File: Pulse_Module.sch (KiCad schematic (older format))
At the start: 6 parts, among them CON3 BARREL_JACK, U3 AP1117

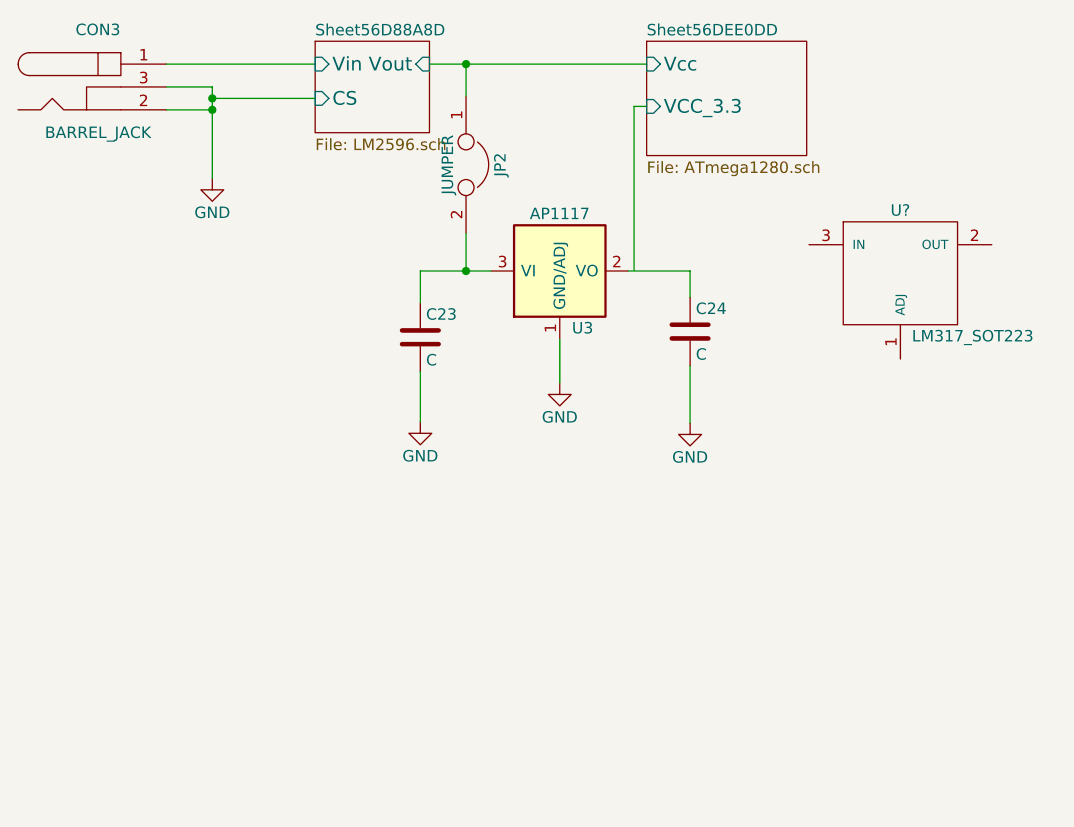
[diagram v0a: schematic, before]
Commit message: Изменения футпринтов
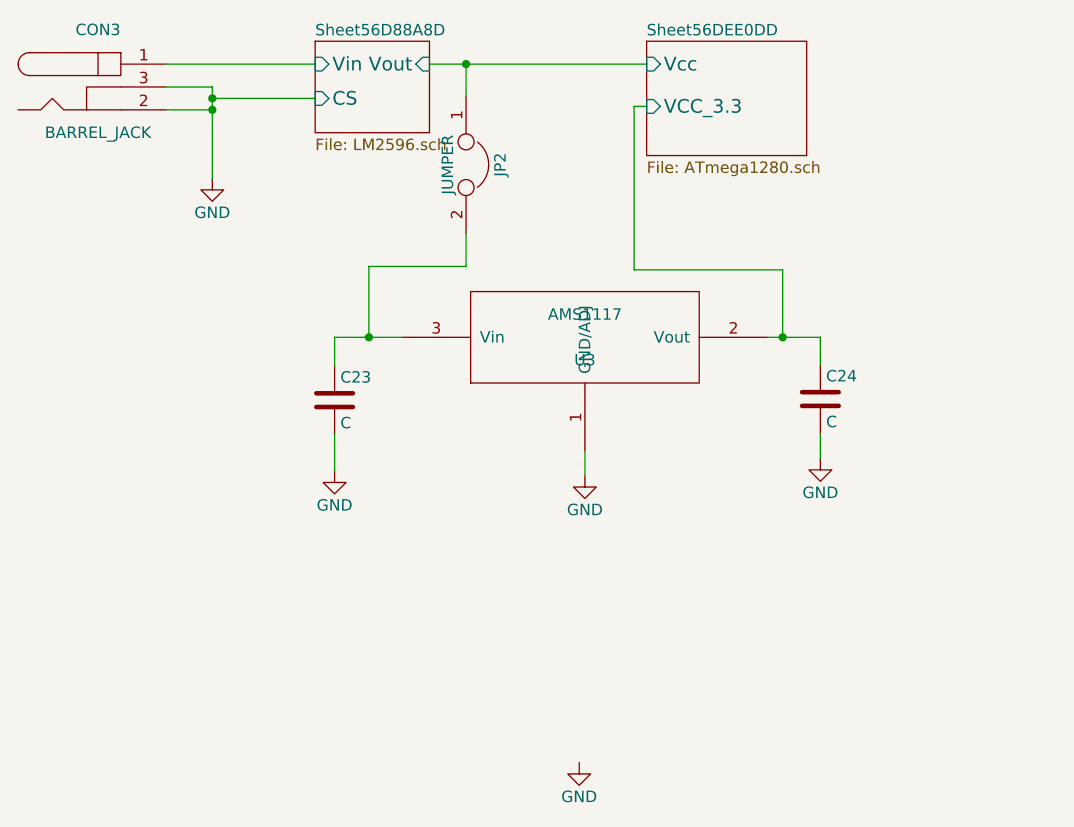
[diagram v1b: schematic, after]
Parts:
- removed U3: AP1117, TO_SOT_Packages_SMD:TO-252-2Lead, symbol AP1117
- removed U?: LM317_SOT223, symbol LM317_SOT223
- added U3: AMS1117, TO_SOT_Packages_SMD:TO-252-2Lead, symbol AMS1117
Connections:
- wire segments 17 -> 21
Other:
- moved on the sheet: C23, C24
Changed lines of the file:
@@
 LIBS:contrib
 LIBS:valves
+LIBS:AMS1117
 LIBS:Pulse_Module-cache
 EELAYER 25 0
@@
 $EndComp
 $Comp
-L AP1117 U3
-U 1 1 57F2F385
-P 4070 4655
-F 0 "U3" H 4170 4405 50  0000 C CNN
-F 1 "AP1117" H 4070 4905 50  0000 C CNN
-F 2 "TO_SOT_Packages_SMD:TO-252-2Lead" H 4070 4655 50  0001 C CNN
-F 3 "" H 4070 4655 50  0000 C CNN
-	1    4070 4655
-	1    0    0    -1
-$EndComp
-$Comp
-L C C23
-U 1 1 57F2F689
-P 3460 4945
-F 0 "C23" H 3485 5045 50  0000 L CNN
-F 1 "C" H 3485 4845 50  0000 L CNN
-F 2 "Capacitors_SMD:C_0805" H 3498 4795 50  0001 C CNN
-F 3 "" H 3460 4945 50  0000 C CNN
-	1    3460 4945
-	1    0    0    -1
-$EndComp
-$Comp
 L C C24
 U 1 1 57F2F6D4
-P 4640 4920
-F 0 "C24" H 4665 5020 50  0000 L CNN
-F 1 "C" H 4665 4820 50  0000 L CNN
-F 2 "Capacitors_SMD:C_0805" H 4678 4770 50  0001 C CNN
-F 3 "" H 4640 4920 50  0000 C CNN
-	1    4640 4920
+P 5210 5215
+F 0 "C24" H 5235 5315 50  0000 L CNN
+F 1 "C" H 5235 5115 50  0000 L CNN
+F 2 "Capacitors_SMD:C_0805" H 5248 5065 50  0001 C CNN
+F 3 "" H 5210 5215 50  0000 C CNN
+	1    5210 5215
 	1    0    0    -1
 $EndComp
@@
 L GND #PWR02
 U 1 1 57F2F7B1
-P 3460 5315
-F 0 "#PWR02" H 3460 5065 50  0001 C CNN
-F 1 "GND" H 3460 5165 50  0000 C CNN
-F 2 "" H 3460 5315 50  0000 C CNN
-F 3 "" H 3460 5315 50  0000 C CNN
-	1    3460 5315
+P 4180 5550
+F 0 "#PWR02" H 4180 5300 50  0001 C CNN
+F 1 "GND" H 4180 5400 50  0000 C CNN
+F 2 "" H 4180 5550 50  0000 C CNN
+F 3 "" H 4180 5550 50  0000 C CNN
+	1    4180 5550
 	1    0    0    -1
 $EndComp
@@
 L GND #PWR03
 U 1 1 57F2F900
-P 4640 5320
-F 0 "#PWR03" H 4640 5070 50  0001 C CNN
-F 1 "GND" H 4640 5170 50  0000 C CNN
-F 2 "" H 4640 5320 50  0000 C CNN
-F 3 "" H 4640 5320 50  0000 C CNN
-	1    4640 5320
+P 5210 5475
+F 0 "#PWR03" H 5210 5225 50  0001 C CNN
+F 1 "GND" H 5210 5325 50  0000 C CNN
+F 2 "" H 5210 5475 50  0000 C CNN
+F 3 "" H 5210 5475 50  0000 C CNN
+	1    5210 5475
 	1    0    0    -1
 $EndComp
@@
 L GND #PWR04
 U 1 1 57F30351
-P 4070 5145
-F 0 "#PWR04" H 4070 4895 50  0001 C CNN
-F 1 "GND" H 4070 4995 50  0000 C CNN
-F 2 "" H 4070 5145 50  0000 C CNN
-F 3 "" H 4070 5145 50  0000 C CNN
-	1    4070 5145
+P 4155 6805
+F 0 "#PWR04" H 4155 6555 50  0001 C CNN
+F 1 "GND" H 4155 6655 50  0000 C CNN
+F 2 "" H 4155 6805 50  0000 C CNN
+F 3 "" H 4155 6805 50  0000 C CNN
+	1    4155 6805
 	1    0    0    -1
 $EndComp
@@
 Wire Wire Line
 	3500 3750 4450 3750
-Wire Wire Line
-	4640 5070 4640 5320
-Wire Wire Line
-	3460 5095 3460 5315
-Connection ~ 3660 4655
 Connection ~ 3660 3750
 Wire Wire Line
-	4070 4955 4070 5145
-Wire Wire Line
-	4370 4655 4640 4655
-Wire Wire Line
-	4640 4655 4640 4770
-Wire Wire Line
-	4395 4650 4395 3935
-Wire Wire Line
 	3660 3750 3660 3890
-Wire Wire Line
-	3460 4655 3460 4795
 $Sheet
 S 4450 3650 700  500
@@
 Wire Wire Line
 	4395 3935 4450 3935
-Wire Wire Line
-	3460 4655 3770 4655
-Wire Wire Line
-	3660 4490 3660 4655
 $Comp
-L LM317_SOT223 U?
-U 1 1 57F44B74
-P 5560 4690
-F 0 "U?" H 5560 4990 50  0000 C CNN
-F 1 "LM317_SOT223" H 5610 4440 50  0000 L CNN
-F 2 "" H 5560 4690 50  0000 C CNN
-F 3 "" H 5560 4690 50  0000 C CNN
-	1    5560 4690
+L AMS1117 U3
+U 1 1 57F689F7
+P 4180 4945
+F 0 "U3" H 4180 4845 50  0000 C CNN
+F 1 "AMS1117" H 4180 5045 50  0000 C CNN
+F 2 "TO_SOT_Packages_SMD:TO-252-2Lead" H 4180 4945 60  0001 C CNN
+F 3 "" H 4180 4945 60  0000 C CNN
+	1    4180 4945
 	1    0    0    -1
 $EndComp
+$Comp
+L C C23
+U 1 1 57F2F689
+P 3085 5220
+F 0 "C23" H 3110 5320 50  0000 L CNN
+F 1 "C" H 3110 5120 50  0000 L CNN
+F 2 "Capacitors_SMD:C_0805" H 3123 5070 50  0001 C CNN
+F 3 "" H 3085 5220 50  0000 C CNN
+	1    3085 5220
+	1    0    0    -1
+$EndComp
+Wire Wire Line
+	3660 4490 3660 4635
+Wire Wire Line
+	3660 4635 3235 4635
+Wire Wire Line
+	3235 4635 3235 4945
+Wire Wire Line
+	3085 4945 3380 4945
+Wire Wire Line
+	3085 4945 3085 5070
+Connection ~ 3235 4945
+$Comp
+L GND #PWR05
+U 1 1 57F69DF6
+P 3085 5530
+F 0 "#PWR05" H 3085 5280 50  0001 C CNN
+F 1 "GND" H 3085 5380 50  0000 C CNN
+F 2 "" H 3085 5530 50  0000 C CNN
+F 3 "" H 3085 5530 50  0000 C CNN
+	1    3085 5530
+	1    0    0    -1
+$EndComp
+Wire Wire Line
+	3085 5370 3085 5530
+Wire Wire Line
+	4180 5445 4180 5550
+Wire Wire Line
+	4980 4945 5210 4945
+Wire Wire Line
+	5210 4945 5210 5065
+Wire Wire Line
+	5210 5365 5210 5475
+Wire Wire Line
+	4395 3935 4395 4650
+Wire Wire Line
+	4395 4650 5045 4650
+Wire Wire Line
+	5045 4650 5045 4945
+Connection ~ 5045 4945
 $EndSCHEMATC
